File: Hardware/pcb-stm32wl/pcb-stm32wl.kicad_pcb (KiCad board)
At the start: 4 copper layers, 40.9 x 67.7 mm, 166 parts, among them J1 Debug, J2 U.FL-R-SMT-1, J3 Grove_I2C, Q1 SI2323DS, Q2 2SC4213, SW1 SW_Push, SW2 RESET, U1 TPS22917DBV, U10 NX3L1T3157GM, U11 BGS13S4N9, U12 NX3L1T3157GM, U2 RP605Z283B, U3 TPS22917DBV, U4 TPS22917DBV, U5 MX25R1635, U6 LIS2DH12, U7 SHTC3, U8 ATECC608A-TNGLORAU, U9 STM32WLxx_QFN48, X1 32MHz, X2 32.768KHz

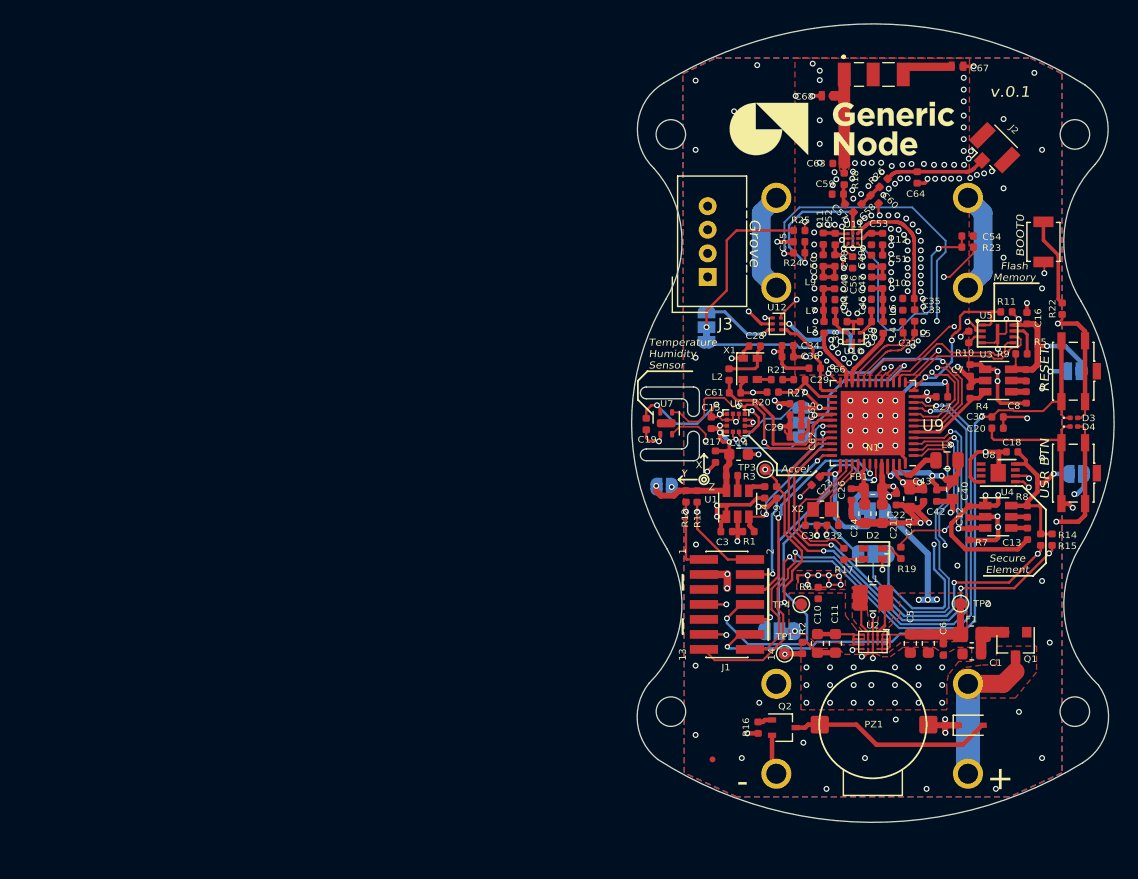
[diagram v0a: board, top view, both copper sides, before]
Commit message: hw: Update latest design files and Readme
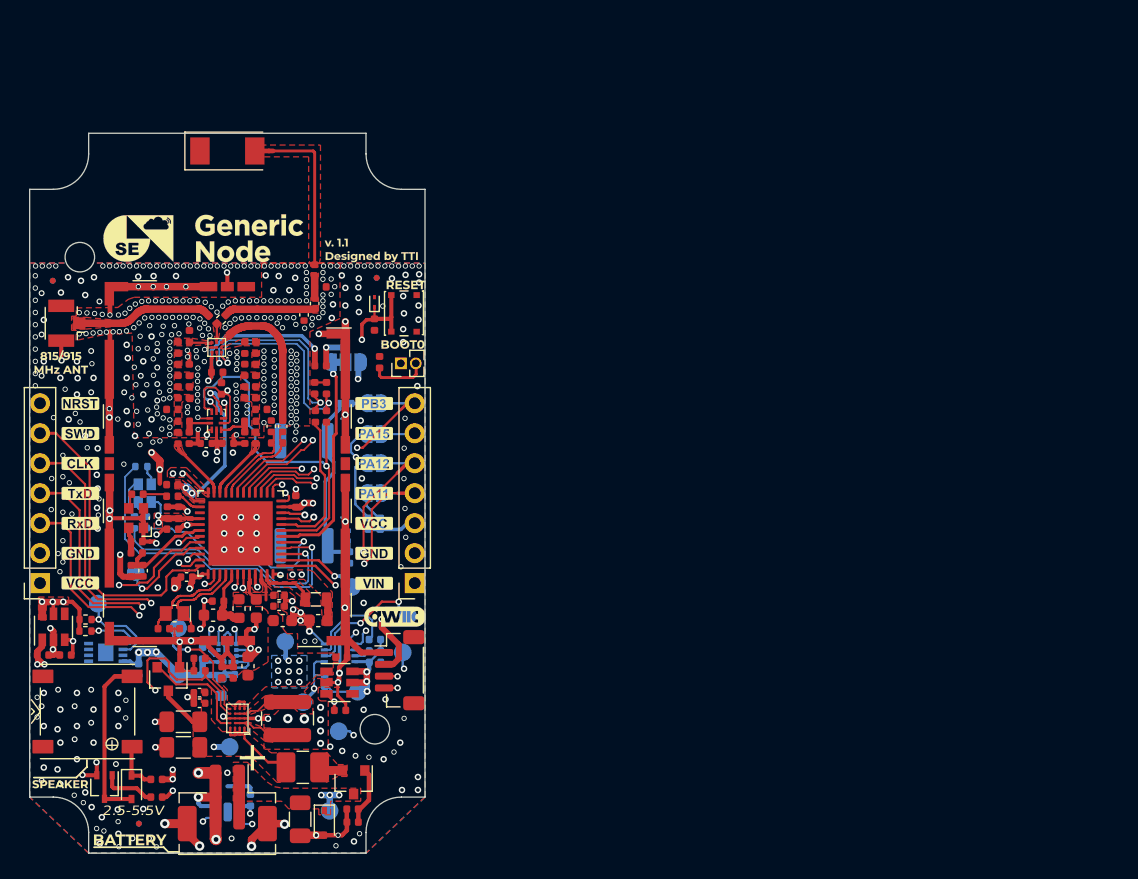
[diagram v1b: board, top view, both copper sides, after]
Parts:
- removed BH1, BH3: Battery_Cell+, node-lib-v1:BAT_BK-92
- removed BH2, BH4: Battery_Cell-, node-lib-v1:BAT_BK-92
- removed C51, C66: 33pF, Capacitor_SMD:C_0402_1005Metric
- removed C52: 2.7pF, Capacitor_SMD:C_0402_1005Metric
- removed C53: 1.3pF, Capacitor_SMD:C_0402_1005Metric
- removed C56: 1nF, Capacitor_SMD:C_0402_1005Metric
- removed C67: 5.0pF, Capacitor_SMD:C_0402_1005Metric
- removed C68: 3.6pF, Capacitor_SMD:C_0402_1005Metric
- removed G***: LOGO, node-lib-v1:qr_azerimaker_11mm
- removed G*** (x2): LOGO, node-lib-v1:Icon_Battery_1000px
- removed G*** (x2): LOGO, node-lib-v1:Logo_GN-4000px
- removed H3, H4: MountingHole, MountingHole:MountingHole_2.5mm
- removed JP10: BOOT0, Button_Switch_SMD:SW_SPST_B3U-1000P
- removed JP11: VDD_RF_SW, Jumper:SolderJumper-3_P1.3mm_Bridged12_RoundedPad1.0x1.5mm_NumberLabels
- removed JP7: VBAT, Jumper:SolderJumper-3_P1.3mm_Bridged12_RoundedPad1.0x1.5mm_NumberLabels
- removed JP8: SWO, Jumper:SolderJumper-3_P1.3mm_Bridged12_RoundedPad1.0x1.5mm_NumberLabels
- removed JP9: INT, Jumper:SolderJumper-3_P1.3mm_Bridged12_RoundedPad1.0x1.5mm_NumberLabels
- removed R25: 100R, Resistor_SMD:R_0402_1005Metric
- removed R26, R27: 0R, Resistor_SMD:R_0402_1005Metric
- removed the REF** at (139.7, 95.5)
- removed the REF** at (147.8, 95.5)
- removed U12: NX3L1T3157GM, node-lib-v1:6-XFDFN_SOT-886
- removed X2: 32.768KHz, node-lib-v1:Crystal_SMD_NX2012SA_32.768KHz
- added D5: ESD9D5V, Diode_SMD:D_SOD-923, F.Cu at (97.5, 88.8)
- added FID2: Fiducial, Fiducial:Fiducial_0.5mm_Mask1.5mm, B.Cu at (77.5, 133.0)
- added FID3: Fiducial, Fiducial:Fiducial_0.5mm_Mask1.5mm, F.Cu at (70.2, 87.0)
- added FID4: Fiducial, Fiducial:Fiducial_0.5mm_Mask1.5mm, B.Cu at (70.2, 87.0)
- added FID5: Fiducial, Fiducial:Fiducial_0.5mm_Mask1.5mm, F.Cu at (97.7, 86.8)
- added FID6: Fiducial, Fiducial:Fiducial_0.5mm_Mask1.5mm, B.Cu at (97.7, 86.8)
- added G-ACCELL: LOGO, node-lib-v1:LAbel_ACCELL_2000px, B.Cu at (83.1, 123.0)
- added G-ANT: LOGO, node-lib-v1:Label_ANT, F.Cu at (71.0, 93.9)
- added G-BAT: LOGO, node-lib-v1:Label_BATTERY_2500px, F.Cu at (76.7, 134.3)
- added G-BOOT0: LOGO, node-lib-v1:Label_BOOT0_4000px, F.Cu at (99.8, 92.3)
- added G-CLK: LOGO, node-lib-v1:PinName_CLK, F.Cu at (72.6, 102.5)
- added G-FLASH: LOGO, node-lib-v1:Label_FLASH_3000px, B.Cu at (92.3, 115.1)
- added G-GND: LOGO, node-lib-v1:PinName_GND, F.Cu at (97.4, 110.1)
- added G-GND2: LOGO, node-lib-v1:PinName_GND, F.Cu at (72.6, 110.1)
- added G-Logo: LOGO, node-lib-v1:Logo_GN-SE-4500px, F.Cu at (83.0, 83.4)
- added G-NRST: LOGO, node-lib-v1:PinName_NRST, F.Cu at (72.6, 97.4)
- added G-PA11: LOGO, node-lib-v1:PinName_PA11, F.Cu at (97.4, 105.0)
- added G-PA12: LOGO, node-lib-v1:PinName_PA12, F.Cu at (97.4, 102.5)
- added G-PA15: LOGO, node-lib-v1:PinName_PA15, F.Cu at (97.4, 99.9)
- added G-PB3: LOGO, node-lib-v1:PinName_PB3, F.Cu at (97.4, 97.4)
- added G-QWIIC: LOGO, node-lib-v1:Logo_qwiic_4000px, F.Cu at (99.2, 115.4)
- added G-RST: LOGO, node-lib-v1:Label_RESET_4000px, F.Cu at (100.1, 87.3)
- added G-RXD: LOGO, node-lib-v1:PinName_RxD, F.Cu at (72.6, 107.5)
- added G-SE: LOGO, node-lib-v1:Label_SE_3000px, B.Cu at (77.0, 115.0)
- added G-SPKR: LOGO, node-lib-v1:Label_Speaker, F.Cu at (70.9, 129.6)
- added G-SWD: LOGO, node-lib-v1:PinName_SWD, F.Cu at (72.6, 99.9)
- added G-TH: LOGO, node-lib-v1:Label_T_H_2000px, B.Cu at (90.0, 128.8)
- added G-TXD: LOGO, node-lib-v1:PinName_TxD, F.Cu at (72.6, 105.0)
- added G-VCC: LOGO, node-lib-v1:PinName_VCC, F.Cu at (97.4, 107.5)
- added G-VCC2: LOGO, node-lib-v1:PinName_VCC, F.Cu at (72.5, 112.6)
- added G-VIN: LOGO, node-lib-v1:PinName_VIN, F.Cu at (97.4, 112.6)
- added G-version: LOGO, node-lib-v1:Logo_design_version_2000px, F.Cu at (97.5, 84.2)
- added J10: Qwiic, Connector_JST:JST_SH_BM04B-SRSS-TB_1x04-1MP_P1.00mm_Vertical, F.Cu at (99.6, 120.0)
- added J4: RF_Shield_One_Piece, node-lib-v1:RF_Shield_SnapOn_30x20mm_w_Cutout_n_GND_Pads, F.Cu at (85.0, 102.5)
- added J5: S1001-46R, node-lib-v1:RF_Shield_Clip_S1001-46R, F.Cu at (85.0, 117.5)
- added J6: S1001-46R, node-lib-v1:RF_Shield_Clip_S1001-46R, F.Cu at (95.0, 102.5)
- added J7: U.FL/iPEX, Connector_Coaxial:U.FL_Hirose_U.FL-R-SMT-1_Vertical, F.Cu at (71.4, 90.6)
- added J8: DEBUG, Connector_PinSocket_2.54mm:PinSocket_1x07_P2.54mm_Vertical, F.Cu at (69.1, 112.6)
- added J9: UART/I2C, Connector_PinSocket_2.54mm:PinSocket_1x07_P2.54mm_Vertical, F.Cu at (100.9, 112.6)
- added JP4: SCL2_CUT, Jumper:SolderJumper-2_P1.3mm_Bridged2Bar_RoundedPad1.0x1.5mm, B.Cu at (97.4, 102.5)
- added JP5: BOOT0, Connector_PinHeader_1.27mm:PinHeader_1x02_P1.27mm_Vertical, F.Cu at (99.7, 94.0)
- added L13: 23nH, Inductor_SMD:L_0402_1005Metric, F.Cu at (92.4, 86.1)
- added L14: 4.3nH, Inductor_SMD:L_0402_1005Metric, F.Cu at (92.9, 87.5)
- added REF**: FabDrawing-4Layer, node-lib-v1:PCBStackup_FabDrawing-4Layer-Metric, F.Cu at (150.0, 72.5)
- added TP10: VCC_F, TestPoint:TestPoint_Pad_D1.5mm, B.Cu at (96.0, 121.8)
- added TP11: VCC_S, TestPoint:TestPoint_Pad_D1.5mm, B.Cu at (80.8, 120.4)
- added TP12: SDA, TestPoint:TestPoint_Pad_D1.5mm, B.Cu at (77.2, 111.7)
- added TP13: SCL, TestPoint:TestPoint_Pad_D1.5mm, B.Cu at (74.0, 114.4)
- added TP5: VCC, TestPoint:TestPoint_Pad_D1.5mm, B.Cu at (89.9, 117.6)
- added TP6: CS, TestPoint:TestPoint_Pad_D1.5mm, B.Cu at (91.4, 122.7)
- added TP7: MISO, TestPoint:TestPoint_Pad_D1.5mm, B.Cu at (100.3, 115.4)
- added TP8: SCK, TestPoint:TestPoint_Pad_D1.5mm, B.Cu at (94.4, 125.2)
- added TP9: MOSI, TestPoint:TestPoint_Pad_D1.5mm, B.Cu at (99.9, 118.5)
- added Y1: 32.768KHz, node-lib-v1:Crystal_SMD_NX2012SA_32.768KHz, F.Cu at (80.5, 115.2)
- AE1: value ANT_M620720 -> NN02-201; footprint node-lib-v1:ANT_M620720 -> node-lib-v1:Antenna_Fractus_NN02-201
- C1: value 10uF -> 100uF; footprint Capacitor_SMD:C_0603_1608Metric -> Capacitor_SMD:C_1206_3216Metric
- C10: value DNM -> 100nF; footprint Capacitor_SMD:C_0603_1608Metric -> Capacitor_SMD:C_0402_1005Metric
- C11: value 22uF -> 1uF; footprint Capacitor_SMD:C_0603_1608Metric -> Capacitor_SMD:C_0402_1005Metric
- C12: value 1uF -> 22uF; footprint Capacitor_SMD:C_0402_1005Metric -> Capacitor_SMD:C_0603_1608Metric
- C13: value DNM -> 4.7uF; footprint Capacitor_SMD:C_0402_1005Metric -> Capacitor_SMD:C_0603_1608Metric
- C14: value 10uF -> 100nF; footprint Capacitor_SMD:C_0603_1608Metric -> Capacitor_SMD:C_0402_1005Metric
- C15, C27: value 100nF -> 4.7uF; footprint Capacitor_SMD:C_0402_1005Metric -> Capacitor_SMD:C_0603_1608Metric
- C19, C22, C42: value 100nF -> 33pF
- C2: value 10uF -> 10nF; footprint Capacitor_SMD:C_0603_1608Metric -> Capacitor_SMD:C_0402_1005Metric
- C20: value DNM -> 100nF
- C21, C41: value 4.7uF -> 33pF; footprint Capacitor_SMD:C_0603_1608Metric -> Capacitor_SMD:C_0402_1005Metric
- C23: value 100nF -> 47pF
- C24: value 4.7uF -> 100nF; footprint Capacitor_SMD:C_0603_1608Metric -> Capacitor_SMD:C_0402_1005Metric
- C25: value 100nF -> 47nF
- C26: value 100nF -> 68pF
- C28: value 10nF -> 470nF; footprint Capacitor_SMD:C_0402_1005Metric -> Capacitor_SMD:C_0603_1608Metric
- C29: value 1nF -> 100nF
- C30, C44: value 6.8pF -> 2.7pF
- C31: value 2.7pF -> 3.6pF
- C32: value 6.8pF -> 33pF
- C33: value 3.6pF -> 33pF
- C34: value 47nF -> 10nF
- C35: value DNM -> 5.6pF
- C36: value 68nF -> 6.8pF
- C37: value 100nF -> 2.7pF
- C38: value 33pF -> 2.4pF
- C39: value 33pF -> 3.3pF
- C4: value DNM -> 100uF; footprint Capacitor_SMD:C_0402_1005Metric -> Capacitor_SMD:C_1206_3216Metric
- C40: value 470nF -> 3.9pF; footprint Capacitor_SMD:C_0603_1608Metric -> Capacitor_SMD:C_0402_1005Metric
- C43: value 100nF -> 1nF
- C45: value 5.6pF -> 1.3pF
- C46: value 2.4pF -> 5.6pF
- C47: value 2.7pF -> 1nF
- C48: value 3.9pF -> 1nF
- C49: value 3.3pF -> 5.6pF
- C5: value 4.7uF -> 100uF; footprint Capacitor_SMD:C_0603_1608Metric -> Capacitor_SMD:C_1206_3216Metric
- C50: value 33pF -> 1nF
- C54: value 1nF -> 3.3pF
- C55: value 1nF -> DNM
- C57, C65: value 33pF -> 100nF
- C58: value DNM -> 10uF; footprint Capacitor_SMD:C_0402_1005Metric -> Capacitor_SMD:C_0603_1608Metric; moved to B.Cu
- C59, C60, C63, C64: value DNM -> 100nF; moved to B.Cu
- C6: value 100nF -> 1uF
- C61, R15, R24: moved to B.Cu
- C62: value 33pF -> 100nF; moved to B.Cu
- C7: value 1uF -> 100nF
- C8: value DNM -> 1uF
- D1: value 1N4148WS -> PESD5V0S1BA
- D2: value EAST1616RGBB2 -> 1N4148WSF-7; footprint node-lib-v1:LED_RGB_0606 -> node-lib-v1:D_SOD-323F_custom
- D3: value ESDALC6V1-1U2 -> FM-B2020RGBA; footprint Diode_SMD:D_0201_0603Metric -> LED_SMD:LED_Cree-PLCC4_2x2mm_CW; moved to B.Cu
- D4: value ESDALC6V1-1U2 -> ESD9D5V; footprint Diode_SMD:D_0201_0603Metric -> Diode_SMD:D_SOD-923; moved to B.Cu
- F1: value PTC 6V 750MA -> PTC 13V 1A; footprint node-lib-v1:Fuse_0805_2012Metric_Castellated -> Fuse:Fuse_1210_3225Metric_Castellated
- J1: value Debug -> S1001-46R; footprint node-lib-v1:PinHeader_2x07_P1.27mm_Vertical_SMD -> node-lib-v1:RF_Shield_Clip_S1001-46R
- J2: value U.FL-R-SMT-1 -> JST-PH; footprint Connector_Coaxial:U.FL_Hirose_U.FL-R-SMT-1_Vertical -> Connector_JST:JST_PH_B2B-PH-SM4-TB_1x02-1MP_P2.00mm_Vertical
- J3: value Grove_I2C -> S1001-46R; footprint Connector:NS-Tech_Grove_1x04_P2mm_Vertical -> node-lib-v1:RF_Shield_Clip_S1001-46R
- JP1: value Sensor_VCC -> VDD_RF_SW; footprint Jumper:SolderJumper-2_P1.3mm_Open_RoundedPad1.0x1.5mm -> Jumper:SolderJumper-3_P1.3mm_Bridged12_RoundedPad1.0x1.5mm_NumberLabels
- JP2: value Flash_VCC -> BUZZ_KILL; footprint Jumper:SolderJumper-2_P1.3mm_Open_RoundedPad1.0x1.5mm -> Jumper:SolderJumper-2_P1.3mm_Bridged2Bar_RoundedPad1.0x1.5mm
- JP3: value Secure_Element_VCC -> SDA2_CUT; footprint Jumper:SolderJumper-2_P1.3mm_Open_RoundedPad1.0x1.5mm -> Jumper:SolderJumper-2_P1.3mm_Bridged2Bar_RoundedPad1.0x1.5mm
- JP6: value JTDI -> BTN_CUT; footprint Jumper:SolderJumper-3_P1.3mm_Bridged12_RoundedPad1.0x1.5mm_NumberLabels -> Jumper:SolderJumper-2_P1.3mm_Bridged2Bar_RoundedPad1.0x1.5mm
- L1: value 2.2 uH -> 2.2uH; footprint Inductor_SMD:L_1008_2520Metric -> node-lib-v1:L_HPC4012TF-2R2M
- L10: value 3.3nH -> 1400R @1GHz
- L2: value 1400R @1GHz -> 3.3nH
- L4: value 3.3nH -> 15uH; footprint Inductor_SMD:L_0402_1005Metric -> node-lib-v1:L_0805_2012Metric_custom
- L8: value 15uH -> 3nH; footprint Inductor_SMD:L_0805_2012Metric -> Inductor_SMD:L_0402_1005Metric
- N1: value NewAge_3inch_round -> BoLink-16174563; footprint node-lib-v1:NewAge_3inch_round -> node-lib-v1:BoLink_704025
- PZ1: value AST0927 2.73kHz 85dB -> MLT-7525; footprint node-lib-v1:Buzzer_AST0927MW-3.6TRQ -> node-lib-v1:Buzzer_MLT-7525
- Q1: value SI2323DS -> CEN2321A
- Q2: value 2SC4213 -> S9013W
- R1: value 100K -> 10K
- R11: value 10K -> DNM; moved to B.Cu
- R12: value 4K7 -> DNM; moved to B.Cu
- R13: value 4K7 -> 10K; moved to B.Cu
- R17: value 330R -> 4K7
- R18: value 0R -> 4K7; moved to B.Cu
- R19: value 100R -> 33R
- R20: value DNM -> 10K
- R21: value 220R -> 1K; footprint Inductor_SMD:L_0402_1005Metric -> Resistor_SMD:R_0402_1005Metric; moved to B.Cu
- R22: value 10K -> 330R; footprint Inductor_SMD:L_0402_1005Metric -> Resistor_SMD:R_0402_1005Metric; moved to B.Cu
- R23: value 100R -> 330R; moved to B.Cu
- R3: value 1K -> 100K
- R5: value 1K -> 220R; footprint Resistor_SMD:R_0402_1005Metric -> Inductor_SMD:L_0402_1005Metric
- R6: value 0R -> 100R
- R7: value 100K -> 100R
- R8: value 1K -> 100R
- R9: value DNM -> 0R
- SW1: value SW_Push -> USR_BTN; footprint node-lib-v1:EVQ-P2R02W -> node-lib-v1:PushButton_KSC721GLFS; moved to B.Cu
- SW2: footprint node-lib-v1:EVQ-P2R02W -> node-lib-v1:SW_SPST_SKSHABE010
- TP1: value VBAT_READ -> VIN; footprint TestPoint:TestPoint_Pad_D1.0mm -> TestPoint:TestPoint_Pad_D1.5mm; moved to B.Cu
- TP2: footprint TestPoint:TestPoint_Pad_D1.0mm -> TestPoint:TestPoint_Pad_D1.5mm; moved to B.Cu
- TP3: value VBAT_ADC -> VBAT_READ_EN; footprint TestPoint:TestPoint_Pad_D1.0mm -> TestPoint:TestPoint_Pad_D1.5mm; moved to B.Cu
- TP4: value VDD -> VBAT_ADC; footprint TestPoint:TestPoint_Pad_D1.0mm -> TestPoint:TestPoint_Pad_D1.5mm; moved to B.Cu
- U10: value NX3L1T3157GM -> SHTC3; footprint node-lib-v1:6-XFDFN_SOT-886 -> node-lib-v1:Sensirion_DFN-4-1EP_2x2mm_P1mm_EP0.7x1.6mm; moved to B.Cu
- U11: value BGS13S4N9 -> ATECC608A-TNGLORA; footprint node-lib-v1:RFSW_BGS13S4N9E6327XTSA1 -> Package_DFN_QFN:DFN-8-1EP_3x2mm_P0.5mm_EP1.3x1.5mm; moved to B.Cu
- U2: value RP605Z283B -> TPS3839G25; footprint node-lib-v1:WLCSP-20-P3_1.994x1.609mm_Layout5x4_P0.4mm -> Package_TO_SOT_SMD:SOT-23
- U4: value TPS22917DBV -> RP605Z283B; footprint Package_TO_SOT_SMD:SOT-23-6 -> node-lib-v1:WLCSP-20-P3_1.994x1.609mm_Layout5x4_P0.4mm
- U5: value MX25R1635 -> STM32WLE5CC; footprint node-lib-v1:FLASH_UFDFN-8-MX25R1635F -> Package_DFN_QFN:QFN-48-1EP_7x7mm_P0.5mm_EP5.45x5.45mm
- U6: value LIS2DH12 -> TS3A5223RSWR; footprint Package_LGA:LGA-12_2x2mm_P0.5mm -> Package_DFN_QFN:UQFN-10_1.4x1.8mm_P0.4mm
- U7: value SHTC3 -> BGS13S4N9; footprint node-lib-v1:Sensirion_DFN-4-1EP_2x2mm_P1mm_EP0.7x1.6mm -> node-lib-v1:RFSW_BGS13S4N9E6327XTSA1
- U8: value ATECC608A-TNGLORAU -> MX25R1635; footprint Package_DFN_QFN:DFN-8-1EP_3x2mm_P0.5mm_EP1.3x1.5mm -> node-lib-v1:FLASH_UFDFN-8-MX25R1635F; moved to B.Cu
- U9: value STM32WLxx_QFN48 -> LIS2DH12; footprint Package_DFN_QFN:QFN-48-1EP_7x7mm_P0.5mm_EP5.45x5.45mm -> Package_LGA:LGA-12_2x2mm_P0.5mm; moved to B.Cu
- X1: footprint node-lib-v1:TCXO_NT2016SA-32M-END4263A -> Crystal:Crystal_SMD_Abracon_ABM10-4Pin_2.5x2.0mm
- moved J2 85.0 mm to (85.0, 131.2), turned to 180 degrees
- moved R14 81.2 mm to (73.0, 115.7), turned to 180 degrees
- moved R22 79.2 mm to (77.7, 102.7), turned to 0 degrees
- moved D3 79.0 mm to (78.0, 105.0), turned to 270 degrees
- moved R5 76.0 mm to (77.4, 105.1), turned to 180 degrees
- moved C16 74.5 mm to (81.5, 112.1), turned to 180 degrees
- moved C63 73.4 mm to (87.0, 131.0), turned to 270 degrees
- moved R23 73.4 mm to (78.2, 107.5), turned to 90 degrees
- moved U11 72.4 mm to (74.7, 118.5), turned to 0 degrees
- moved C18 71.8 mm to (79.9, 106.6), turned to 90 degrees
- moved C7 71.1 mm to (82.6, 122.8), turned to 180 degrees
- moved R9 67.9 mm to (84.5, 90.3), turned to 225 degrees
- moved C58 67.5 mm to (84.5, 121.4), turned to 90 degrees
- moved L10 67.2 mm to (77.3, 110.1), turned to 180 degrees
- moved U4 66.7 mm to (85.8, 124.1), turned to 90 degrees
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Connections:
- AE1 pad 1: Net-(AE1-Pad1) -> (no net)
- C1 pad 2: Net-(C1-Pad2) -> Vin
- C10 pad 2: Net-(C10-Pad2) -> VDDRF
- C11 pad 1: GND -> VDDRF
- C11 pad 2: Net-(C10-Pad2) -> GND
- C12 pad 1: VDD -> GND
- C12 pad 2: GND -> VDDRF
- C13 pad 1: VDD -> VDDRF
- C13 pad 2: Net-(C13-Pad2) -> GND
- C14 pad 1: GND -> VDDRF
- C14 pad 2: /Peripherals/VCC_SENSORS -> GND
- C15 pad 1: GND -> VDDA
- C15 pad 2: /Peripherals/VCC_SENSORS -> GND
- C16 pad 1: GND -> VDDRF
- C16 pad 2: /Peripherals/VCC_FLASH -> GND
- C17 pad 1: GND -> VDDA
- C17 pad 2: /Peripherals/VCC_SENSORS -> GND
- C18 pad 1: GND -> VDDRF
- C18 pad 2: /Peripherals/VCC_SEC_ELM -> GND
- C19 pad 1: GND -> VDDRF
- C19 pad 2: /Peripherals/VCC_SENSORS -> GND
- C2 pad 1: GND -> Net-(C2-Pad1)
- C2 pad 2: +BATT -> GND
- C20 pad 1: GND -> VDDRF
- C20 pad 2: /LoRa MCU/PB3 -> GND
- C21 pad 1: VDD -> VDDPA
- C22 pad 1: VDD -> VDDRF1V55
- C23 pad 1: Net-(C23-Pad1) -> PB0_VDD_TCXO
- C24 pad 1: VDDA -> PB0_VDD_TCXO
- C25 pad 1: VDDRF -> GND
- C25 pad 2: GND -> Net-(C25-Pad2)
- C26 pad 1: VDDA -> Net-(C25-Pad2)
- C27 pad 1: VDD -> VDDRF
- C28 pad 1: GND -> VDDRF1V55
- C28 pad 2: Net-(C28-Pad2) -> GND
- C29 pad 1: Net-(C29-Pad1) -> VDDRF
- C29 pad 2: OSC_IN -> GND
- C3 pad 1: VDD -> VDDRF
- C30 pad 2: OSC32_IN -> /LoRa MCU/RFI_N
- C31 pad 1: GND -> /LoRa MCU/RFI_P
- C32 pad 2: OSC32_OUT -> Net-(C32-Pad2)
- C33 pad 1: /LoRa MCU/RFI_P -> Net-(C33-Pad1)
- C33 pad 2: Net-(C33-Pad2) -> GND
- C35 pad 1: Net-(C33-Pad2) -> GND
- C35 pad 2: GND -> Net-(C35-Pad2)
- C36 pad 1: Net-(C34-Pad2) -> GND
- C36 pad 2: GND -> Net-(C36-Pad2)
- C37 pad 1: GND -> Net-(C35-Pad2)
- C37 pad 2: NRST -> Net-(C37-Pad2)
- C38 pad 1: GND -> Net-(C36-Pad2)
- C39 pad 1: Net-(C39-Pad1) -> GND
- C39 pad 2: GND -> Net-(C37-Pad2)
- C4 pad 1: VDD -> GND
- C4 pad 2: Net-(C4-Pad2) -> +BATT
- C40 pad 1: VDDRF1V55 -> GND
- C40 pad 2: GND -> Net-(C38-Pad2)
- C41 pad 1: VDDRF -> Net-(C38-Pad2)
- C41 pad 2: GND -> Net-(C41-Pad2)
- C42 pad 1: VDDRF1V55 -> Net-(C37-Pad2)
- C42 pad 2: GND -> Net-(C42-Pad2)
- C43 pad 1: VDDRF -> Net-(C43-Pad1)
- C43 pad 2: GND -> OSC_IN
- C46 pad 1: Net-(C44-Pad2) -> GND
- C46 pad 2: Net-(C46-Pad2) -> OSC32_IN
- C47 pad 1: Net-(C45-Pad2) -> GND
- C48 pad 2: Net-(C46-Pad2) -> Net-(C48-Pad2)
- C49 pad 2: Net-(C47-Pad2) -> OSC32_OUT
- C5 pad 1: +BATT -> GND
- C5 pad 2: GND -> +BATT
- C50 pad 1: Net-(C46-Pad2) -> GND
- C54 pad 1: GND -> Net-(C54-Pad1)
- C55 pad 2: Net-(C55-Pad2) -> Net-(C54-Pad2)
- C57 pad 1: Net-(C57-Pad1) -> VDDRF
- C57 pad 2: Net-(C57-Pad2) -> GND
- C58 pad 1: Net-(C57-Pad1) -> GND
- C58 pad 2: Net-(C58-Pad2) -> /Peripherals/VCC_SENSORS
- C59 pad 2: Net-(C57-Pad2) -> /Peripherals/VCC_SENSORS
- C60 pad 2: Net-(C58-Pad2) -> /Peripherals/VCC_FLASH
- C61 pad 1: PB0_VDD_TCXO -> GND
- C61 pad 2: GND -> /Peripherals/VCC_SENSORS
- C62 pad 1: VDDRF1V55 -> GND
- C62 pad 2: GND -> /Peripherals/VCC_SENSORS
- C63 pad 2: Net-(AE1-Pad1) -> /Peripherals/VCC_SENSORS
- C65 pad 1: VDDRF -> GND
- C65 pad 2: GND -> /LoRa MCU/NRST
- C7 pad 1: VDD -> +BATT
- C8 pad 1: VDD -> VDDRF
- C8 pad 2: Net-(C8-Pad2) -> GND
- D1 pad 1: VDD -> Vin
- D1 pad 2: Net-(D1-Pad2) -> GND
- D3 pad 1: NRST -> Net-(D3-Pad1)
- D3 pad 2: GND -> Net-(D3-Pad2)
- D4 pad 1: /LoRa MCU/PB3 -> Net-(C64-Pad2)
- F1 pad 2: Net-(C1-Pad2) -> Net-(F1-Pad2)
- FB1 pad 2: VDD -> VDDRF
- J1 pad 1: /LoRa MCU/I2C1_SDA -> GND
- J2 pad 1: Net-(C64-Pad2) -> Vin
- J3 pad 1: /LoRa MCU/I2C1_SCL -> GND
- JP1 pad 1: VDD -> FE_CTRL3
- JP1 pad 2: /Peripherals/VCC_SENSORS -> Net-(JP1-Pad2)
- JP2 pad 1: VDD -> /LoRa MCU/PA15
- JP2 pad 2: /Peripherals/VCC_FLASH -> Net-(JP2-Pad2)
- JP3 pad 1: VDD -> Net-(JP3-Pad1)
- JP3 pad 2: /Peripherals/VCC_SEC_ELM -> /LoRa MCU/PA11_SDA2
- JP6 pad 1: /Peripherals/BUZZER -> /LoRa MCU/PB3
- L10 pad 1: Net-(C45-Pad2) -> PB0_VDD_TCXO
- L10 pad 2: Net-(C47-Pad2) -> Net-(C34-Pad2)
- L11 pad 1: Net-(C50-Pad2) -> Net-(C41-Pad2)
- L11 pad 2: Net-(C52-Pad2) -> Net-(C44-Pad2)
- L12 pad 1: Net-(C51-Pad2) -> Net-(C42-Pad2)
- L12 pad 2: Net-(C53-Pad2) -> Net-(C45-Pad2)
- L2 pad 1: PB0_VDD_TCXO -> Net-(L2-Pad1)
- L2 pad 2: Net-(C28-Pad2) -> Net-(C35-Pad2)
- L3 pad 2: Net-(C44-Pad2) -> Net-(C36-Pad2)
- L4 pad 1: Net-(L4-Pad1) -> VLXSMPS
- L4 pad 2: Net-(C45-Pad2) -> VDDRF1V55
- L5 pad 1: Net-(C31-Pad2) -> /LoRa MCU/RFI_N
- L6 pad 1: Net-(C39-Pad1) -> Net-(C32-Pad2)
- L6 pad 2: Net-(C45-Pad2) -> Net-(C36-Pad2)
- L7 pad 1: Net-(C38-Pad2) -> Net-(C33-Pad1)
- L7 pad 2: Net-(C44-Pad2) -> Net-(C35-Pad2)
- L8 pad 1: VLXSMPS -> Net-(C35-Pad2)
- L8 pad 2: VDDRF1V55 -> Net-(C37-Pad2)
- L9 pad 1: Net-(C44-Pad2) -> Net-(C36-Pad2)
- L9 pad 2: Net-(C46-Pad2) -> Net-(C38-Pad2)
- PZ1 pad 1: VDD -> Net-(D2-Pad1)
- PZ1 pad 2: Net-(D1-Pad2) -> Net-(D2-Pad2)
- Q1 pad 1: GND -> Net-(C2-Pad1)
- Q1 pad 2: Net-(C1-Pad2) -> Net-(F1-Pad2)
- Q1 pad 3: Net-(BH1-Pad1) -> Vin
- Q2 pad 3: Net-(D1-Pad2) -> Net-(D2-Pad2)
- R1 pad 2: /LoRa MCU/PB12 -> Net-(C2-Pad1)
- R10 pad 1: /Peripherals/VCC_FLASH -> Net-(J7-Pad1)
- R11 pad 2: /Peripherals/FlashCS -> Net-(R11-Pad2)
- R12 pad 1: /LoRa MCU/I2C1_SDA -> /Peripherals/VCC_FLASH
- R12 pad 2: /Peripherals/VCC_SENSORS -> Net-(R12-Pad2)
- R13 pad 1: /Peripherals/VCC_SENSORS -> /Peripherals/VCC_FLASH
- R13 pad 2: /LoRa MCU/I2C1_SCL -> /Peripherals/FlashCS
- R14 pad 1: /LoRa MCU/I2C2_SCL -> /LoRa MCU/PA09_SCL1
- R14 pad 2: /Peripherals/VCC_SEC_ELM -> /Peripherals/VCC_SENSORS
- R15 pad 1: /Peripherals/VCC_SEC_ELM -> Net-(JP3-Pad1)
- R15 pad 2: /LoRa MCU/I2C2_SDA -> VDDRF
- R16 pad 1: /Peripherals/BUZZER -> Net-(JP2-Pad2)
- R17 pad 1: Net-(D2-Pad1) -> /Peripherals/VCC_SENSORS
- R17 pad 2: /Peripherals/LED_R -> /LoRa MCU/PA10_SDA1
- R18 pad 1: Net-(AE1-Pad1) -> VDDRF
- R18 pad 2: Net-(C57-Pad2) -> Net-(JP4-Pad1)
- R19 pad 1: Net-(D2-Pad3) -> VDDRF
- R19 pad 2: /Peripherals/LED_B -> Net-(D2-Pad1)
- R2 pad 2: /LoRa MCU/PB4 -> /Power Supply/LS1_SENSORS_EN
- R20 pad 1: OSC_IN -> GND
- R20 pad 2: GND -> /LoRa MCU/BOOT0
- R21 pad 1: Net-(C29-Pad1) -> /LoRa MCU/PB5
- R21 pad 2: Net-(R21-Pad2) -> Net-(D3-Pad1)
- R22 pad 1: GND -> /LoRa MCU/PB6
- R22 pad 2: Net-(JP10-Pad2) -> Net-(D3-Pad4)
- R23 pad 1: Net-(C54-Pad2) -> /LoRa MCU/PB7
- R23 pad 2: FE_CTRL1 -> Net-(D3-Pad2)
- R24 pad 1: Net-(C55-Pad2) -> Net-(JP6-Pad2)
- R24 pad 2: FE_CTRL2 -> Net-(C64-Pad2)
- R3 pad 1: /Peripherals/VCC_SENSORS -> GND
- R3 pad 2: Net-(R3-Pad2) -> /LoRa MCU/PB4
- R4 pad 2: /LoRa MCU/PB7 -> /Power Supply/LS2_FLASH_EN
- R5 pad 1: /Peripherals/VCC_FLASH -> Net-(C43-Pad1)
- R6 pad 1: Net-(C10-Pad2) -> Net-(C47-Pad2)
- R6 pad 2: VDD -> FE_CTRL2
- R7 pad 1: GND -> Net-(C48-Pad2)
- R7 pad 2: /LoRa MCU/PB6 -> FE_CTRL1
- R8 pad 1: /Peripherals/VCC_SEC_ELM -> Net-(JP1-Pad2)
- R8 pad 2: Net-(R8-Pad2) -> Net-(C50-Pad2)
- R9 pad 1: /Peripherals/VCC_FLASH -> Net-(C54-Pad2)
- R9 pad 2: Net-(R9-Pad2) -> Net-(R10-Pad2)
- SW1 pad 1: GND -> Net-(C64-Pad2)
- SW1 pad 2: /LoRa MCU/PB3 -> GND
- SW2 pad 2: NRST -> /LoRa MCU/NRST
- TP1 pad 1: /LoRa MCU/PB4 -> Vin
- TP3 pad 1: /LoRa MCU/PB2 -> /LoRa MCU/PB4
- TP4 pad 1: Net-(C10-Pad2) -> /LoRa MCU/PB2
- U1 pad 1: VDD -> VDDRF
- U1 pad 3: /LoRa MCU/PB12 -> /Power Supply/LS1_SENSORS_EN
- U1 pad 4: Net-(C4-Pad2) -> (no net)
- U1 pad 5: Net-(R3-Pad2) -> /Peripherals/VCC_SENSORS
- U10 pad 1: Net-(C39-Pad1) -> /Peripherals/VCC_SENSORS
- U10 pad 2: GND -> /LoRa MCU/PA09_SCL1
- U10 pad 3: Net-(C38-Pad2) -> /LoRa MCU/PA10_SDA1
- U10 pad 4: Net-(C34-Pad2) -> GND
- U10 pad 5: VDD -> (no net)
- U11 pad 1: Net-(C54-Pad2) -> (no net)
- U11 pad 2: Net-(C53-Pad2) -> (no net)
- U11 pad 3: Net-(C33-Pad2) -> (no net)
- U11 pad 4: Net-(C57-Pad1) -> GND
- U11 pad 5: Net-(C52-Pad2) -> /LoRa MCU/PA10_SDA1
- U11 pad 6: GND -> /LoRa MCU/PA09_SCL1
- U11 pad 7: Net-(C56-Pad2) -> (no net)
- U11 pad 8: Net-(C55-Pad2) -> /Peripherals/VCC_SENSORS
- U3 pad 1: VDD -> VDDRF
- U3 pad 3: /LoRa MCU/PB7 -> /Power Supply/LS2_FLASH_EN
- U3 pad 4: Net-(C8-Pad2) -> (no net)
- U3 pad 5: Net-(R5-Pad2) -> /Peripherals/VCC_FLASH
- U5 pad 1: /Peripherals/FlashCS -> /LoRa MCU/PB3
- U5 pad 2: /Peripherals/MISO -> /LoRa MCU/PB4
- U5 pad 3: Net-(R10-Pad2) -> /LoRa MCU/PB5
- U5 pad 4: GND -> /LoRa MCU/PB6
- U5 pad 5: /Peripherals/MOSI -> /LoRa MCU/PB7
- U5 pad 6: /Peripherals/SCLK -> FE_CTRL3
- U5 pad 7: Net-(R9-Pad2) -> FE_CTRL1
- U5 pad 8: /Peripherals/VCC_FLASH -> FE_CTRL2
- U5 pad 9: GND -> /LoRa MCU/PA2_TxD2
- U6 pad 1: /LoRa MCU/I2C1_SCL -> VDDRF
- U6 pad 10: /Peripherals/VCC_SENSORS -> Net-(C33-Pad1)
- U6 pad 2: /Peripherals/VCC_SENSORS -> VDDRF1V55
- U6 pad 3: /Peripherals/VCC_SENSORS -> VDDPA
- U6 pad 4: /LoRa MCU/I2C1_SDA -> FE_CTRL1
- U6 pad 5: GND -> VDDRF
- U6 pad 7: GND -> Net-(C32-Pad2)
- U6 pad 8: GND -> FE_CTRL1
- U6 pad 9: /Peripherals/VCC_SENSORS -> Net-(C25-Pad2)
- U7 pad 1: /Peripherals/VCC_SENSORS -> Net-(C48-Pad2)
- U7 pad 2: /LoRa MCU/I2C1_SCL -> Net-(C45-Pad2)
- U7 pad 3: /LoRa MCU/I2C1_SDA -> Net-(C31-Pad2)
- U7 pad 4: GND -> Net-(R10-Pad2)
- U7 pad 5: Net-(U7-Pad5) -> Net-(C44-Pad2)
- U8 pad 1: (no net) -> /Peripherals/FlashCS
- U8 pad 2: (no net) -> /Peripherals/MISO
- U8 pad 3: (no net) -> Net-(R12-Pad2)
- U8 pad 5: /LoRa MCU/I2C2_SDA -> /Peripherals/MOSI
- U8 pad 6: /LoRa MCU/I2C2_SCL -> /LoRa MCU/PA5_SCK1
- U8 pad 7: (no net) -> Net-(R11-Pad2)
- U8 pad 8: /Peripherals/VCC_SEC_ELM -> /Peripherals/VCC_FLASH
- U9 pad 1: Net-(JP8-Pad2) -> /LoRa MCU/PA09_SCL1
- U9 pad 10: /LoRa MCU/USART2_RxD -> /Peripherals/VCC_SENSORS
- U9 pad 11: VDD -> /LoRa MCU/PA8
- U9 pad 12: /Peripherals/FlashCS -> (no net)
- U9 pad 2: /LoRa MCU/PB4 -> /Peripherals/VCC_SENSORS
- U9 pad 3: /Peripherals/LED_B -> /Peripherals/VCC_SENSORS
- U9 pad 4: /LoRa MCU/PB6 -> /LoRa MCU/PA10_SDA1
- U9 pad 5: /LoRa MCU/PB7 -> GND
- U9 pad 6: FE_CTRL3 -> GND
- U9 pad 7: FE_CTRL1 -> GND
- U9 pad 8: FE_CTRL2 -> GND
- U9 pad 9: /LoRa MCU/USART2_TxD -> /Peripherals/VCC_SENSORS
- X1 pad 3: Net-(R21-Pad2) -> Net-(R5-Pad2)
- X1 pad 4: Net-(C28-Pad2) -> Net-(C34-Pad2)
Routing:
- net VDD: track 179.8 -> 0.00 mm, vias 29 -> 0
- net VDDRF: track 46.7 -> 166.3 mm, vias 5 -> 22
- net /LoRa MCU/PA09_SCL1: track 0.00 -> 72.8 mm, vias 0 -> 5
- net /LoRa MCU/I2C1_SCL: track 69.9 -> 0.00 mm, vias 4 -> 0
- net NRST: track 69.3 -> 0.00 mm, vias 3 -> 0
- net /LoRa MCU/PA12_SCL2: track 0.00 -> 57.1 mm, vias 0 -> 3
- net /LoRa MCU/NRST: track 0.00 -> 56.6 mm, vias 0 -> 2
- net /LoRa MCU/USART2_TxD: track 54.2 -> 0.00 mm, vias 2 -> 0
- net /LoRa MCU/I2C1_SDA: track 53.2 -> 0.00 mm, vias 3 -> 0
- net Net-(BH2-Pad1): track 51.8 -> 0.00 mm
- net /LoRa MCU/PA10_SDA1: track 0.00 -> 51.2 mm, vias 0 -> 4
- net Net-(JP2-Pad2): track 0.00 -> 50.6 mm, vias 0 -> 3
- net /LoRa MCU/USART2_RxD: track 50.5 -> 0.00 mm, vias 2 -> 0
- net /LoRa MCU/PA11_SDA2: track 0.00 -> 50.4 mm, vias 0 -> 3
- net /LoRa MCU/I2C2_SDA: track 48.5 -> 0.00 mm, vias 4 -> 0
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- added copper zone on F.Cu, net /Peripherals/VCC_SENSORS
- added copper zone on In1.LF, net GND
- added copper zone on In2.PWR, net GND
- added copper zone on F.Cu, net Net-(AE1-Pad2)
- added copper zone on F.Cu, net Net-(C25-Pad2)
- added copper zone on F.Cu, net Net-(C31-Pad2)
- added copper zone on F.Cu, net Net-(C35-Pad2)
- added copper zone on F.Cu, net Net-(C36-Pad2)
- added copper zone on F.Cu, net Net-(C37-Pad2)
- added copper zone on F.Cu, net Net-(C38-Pad2)
- added copper zone on F.Cu, net Net-(C41-Pad2)
- added copper zone on F.Cu, net Net-(C42-Pad2)
- added copper zone on F.Cu, net Net-(C44-Pad2)
- added copper zone on F.Cu, net Net-(C45-Pad2)
- added copper zone on F.Cu, net Net-(C54-Pad1)
- added copper zone on F.Cu, net Net-(C54-Pad2)
- added copper zone on F.Cu, net Net-(F1-Pad2)
- added copper zone on F.Cu, net Net-(J7-Pad1)
- added copper zone on F.Cu, net Net-(L2-Pad1)
- added copper zone on F.Cu, net Net-(L3-Pad1)
- added copper zone on F.Cu, net Net-(R10-Pad2)
- added copper zone on F.Cu, net VDDPA
- added copper zone on B.Cu, net VDDRF
- added copper zone on F.Cu, net VDDRF
- added copper zone on In2.PWR, net VDDRF
- added copper zone on F.Cu, net VDDRF1V55
- added copper zone on F.Cu, net VLXSMPS
- added copper zone on F.Cu, net Vin
- removed copper zone on In1.GND, net GND
- removed copper zone on F.Cu, net Net-(AE1-Pad1)
- removed copper zone on F.Cu, net Net-(BH1-Pad1)
- removed copper zone on In2.PWR, net Net-(BH2-Pad1)
- removed copper zone on F.Cu, net Net-(C10-Pad2)
- removed copper zone on F.Cu, net VDD
- removed copper zone on In2.PWR, net VDD
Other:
- board size 40.9 x 67.7 mm -> 33.5 x 61 mm
- rule pad_to_mask_clearance: 0.05 -> 0
- rule trace_min: 0.127 -> 0.1
- rule via_min_drill: 0.2 -> 0.3
- board text added: "1. Material: 2. Soldermask color: 3. Silkscreen color: 4. Surface Finish: 5. Impedance Control: 6. VIAs: 7. Stackup:"
- board text added: "2.5-5.5V"
- board text added: "BUTTON"
- board text added: "CLK"
- board text added: "FR-4 (TG-150) Black/Blue White ENIG Yes Tented with soldermask See stackup table below for layer specific info"
- board text added: "GND"
- board text added: "LED"
- board text added: "NRST"
- board text added: "PA11"
- board text added: "PA12"
- board text added: "PA15"
- board text added: "PB3"
- board text added: "RXD"
- board text added: "SWD"
- board text added: "TXD"
- board text added: "VCC"
- board text added: "VIN"
- board text added: "~PCB Specifications"
- board text removed: "-"
- board text removed: "1.5V-AA"
- board text removed: "Accel."
- board text removed: "BOOT0"
- board text removed: "Flash Memory"
- board text removed: "Grove"
- board text removed: "RESET"
- board text removed: "Secure Element"
- board text removed: "Temperature Humidity Sensor"
- board text removed: "USR BTN"
- board text removed: "v.0.1"
